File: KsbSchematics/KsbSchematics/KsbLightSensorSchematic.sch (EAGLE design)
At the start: 30 parts, among them IC1 7805L, IC2 LM311N, U1 ATTINY84

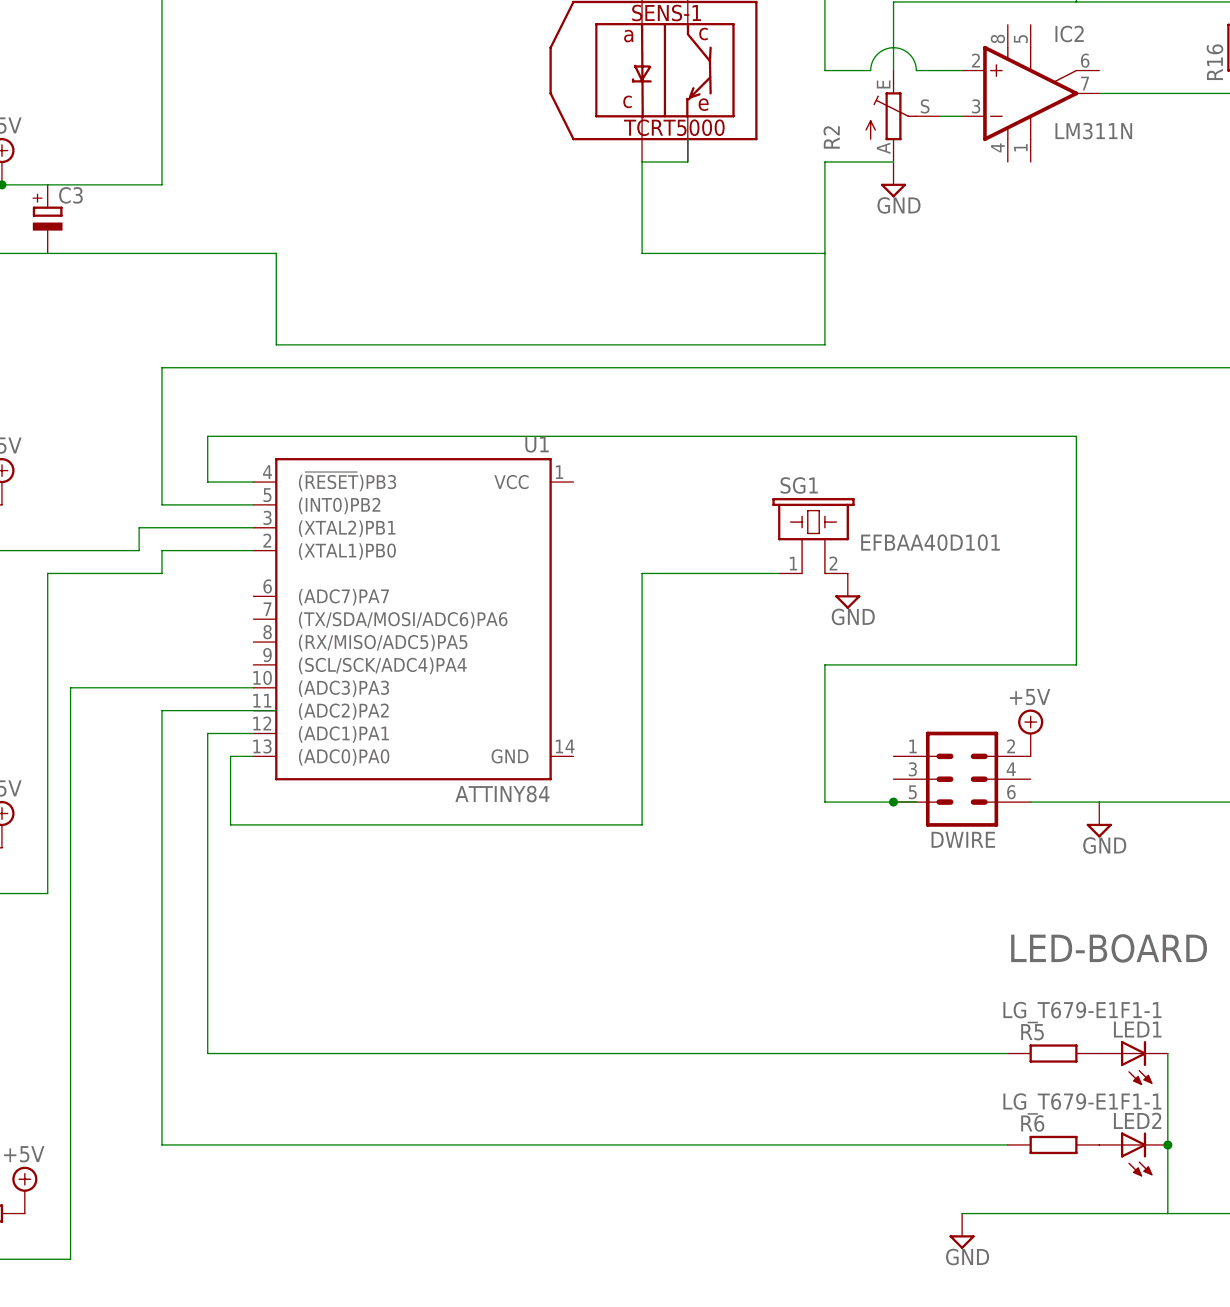
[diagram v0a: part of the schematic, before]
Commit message: schematic changes
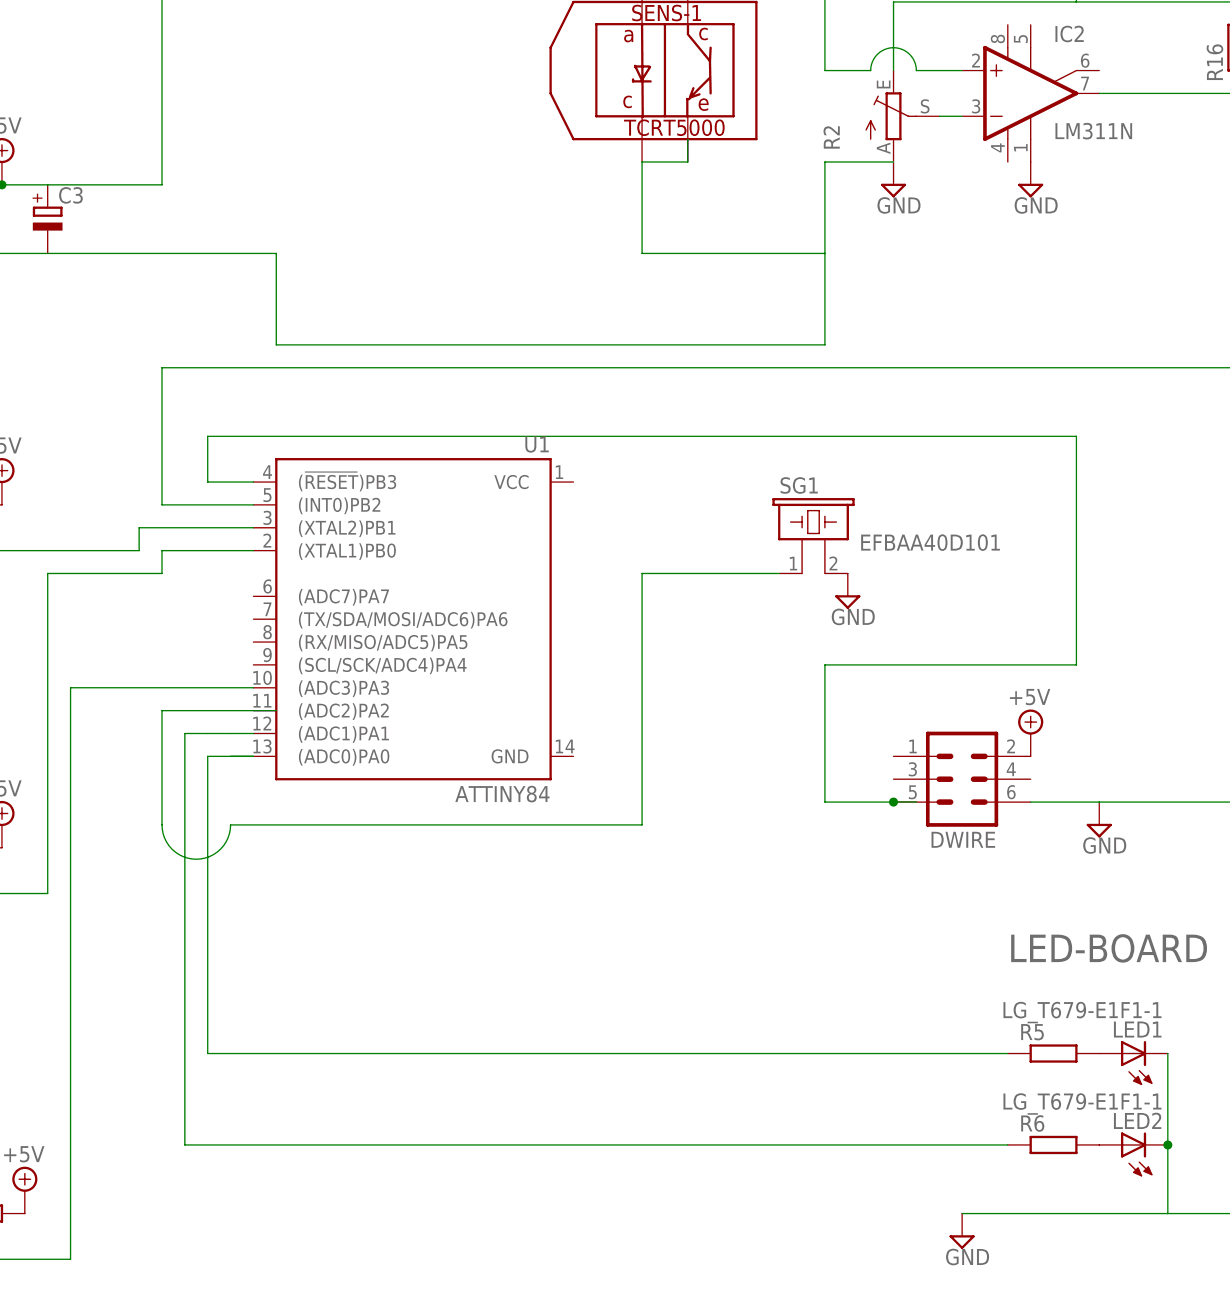
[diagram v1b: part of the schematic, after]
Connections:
- removed net N$10: R6.1
- removed net N$19: SG1.1, U1.(ADC0)PA0
- new net N$12: R6.1, U1.(ADC1)PA1
- new net N$14: SG1.1
- net GND: now also IC2.GND
- net LED-BOARD: now also U1.(ADC0)PA0; no longer U1.(ADC1)PA1
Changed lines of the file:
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@@
 <part name="R7" library="resistor" deviceset="R-EU_" device="0613/5V" value="2k"/>
 <part name="R8" library="resistor" deviceset="R-EU_" device="0613/5V" value="2k"/>
+<part name="SUPPLY26" library="supply2" deviceset="GND" device=""/>
 </parts>
 <sheets>
@@
 <instance part="R7" gate="G$1" x="132.08" y="157.48"/>
 <instance part="R8" gate="G$1" x="132.08" y="149.86"/>
+<instance part="SUPPLY26" gate="GND" x="132.08" y="124.46"/>
 </instances>
 <busses>
@@
 <pinref part="SUPPLY17" gate="GND" pin="GND"/>
 </segment>
+<segment>
+<pinref part="IC2" gate="A" pin="GND"/>
+<pinref part="SUPPLY26" gate="GND" pin="GND"/>
+</segment>
 </net>
 <net name="N$6" class="0">
@@
 </segment>
 </net>
-<net name="N$10" class="0">
-<segment>
-<wire x1="35.56" y1="17.78" x2="129.54" y2="17.78" width="0.1524" layer="91"/>
-<pinref part="R6" gate="G$1" pin="1"/>
-<wire x1="35.56" y1="17.78" x2="35.56" y2="66.04" width="0.1524" layer="91"/>
-<wire x1="35.56" y1="66.04" x2="48.26" y2="66.04" width="0.1524" layer="91"/>
-</segment>
-</net>
 <net name="LED-BOARD" class="0">
 <segment>
@@
 <pinref part="R5" gate="G$1" pin="1"/>
 <label x="129.54" y="38.1" size="3.048" layer="95"/>
-<wire x1="40.64" y1="27.94" x2="40.64" y2="63.5" width="0.1524" layer="91"/>
-<pinref part="U1" gate="U1" pin="(ADC1)PA1"/>
-<wire x1="40.64" y1="63.5" x2="45.72" y2="63.5" width="0.1524" layer="91"/>
+<wire x1="40.64" y1="27.94" x2="40.64" y2="60.96" width="0.1524" layer="91"/>
+<pinref part="U1" gate="U1" pin="(ADC0)PA0"/>
+<wire x1="43.18" y1="60.96" x2="45.72" y2="60.96" width="0.1524" layer="91"/>
+<wire x1="40.64" y1="60.96" x2="45.72" y2="60.96" width="0.1524" layer="91"/>
 </segment>
 </net>
@@
 <pinref part="S2" gate="1" pin="O"/>
 <label x="-76.2" y="50.8" size="2.54" layer="95" rot="R180"/>
-</segment>
-</net>
-<net name="N$19" class="0">
-<segment>
-<pinref part="SG1" gate="G$1" pin="1"/>
-<wire x1="104.14" y1="81.28" x2="88.9" y2="81.28" width="0.1524" layer="91"/>
-<wire x1="88.9" y1="81.28" x2="88.9" y2="53.34" width="0.1524" layer="91"/>
-<wire x1="88.9" y1="53.34" x2="43.18" y2="53.34" width="0.1524" layer="91"/>
-<wire x1="43.18" y1="53.34" x2="43.18" y2="60.96" width="0.1524" layer="91"/>
-<pinref part="U1" gate="U1" pin="(ADC0)PA0"/>
-<wire x1="43.18" y1="60.96" x2="45.72" y2="60.96" width="0.1524" layer="91"/>
 </segment>
 </net>
@@
 </segment>
 </net>
+<net name="N$12" class="0">
+<segment>
+<pinref part="U1" gate="U1" pin="(ADC1)PA1"/>
+<wire x1="38.1" y1="63.5" x2="40.64" y2="63.5" width="0.1524" layer="91"/>
+<pinref part="R6" gate="G$1" pin="1"/>
+<wire x1="43.18" y1="63.5" x2="45.72" y2="63.5" width="0.1524" layer="91"/>
+<wire x1="129.54" y1="17.78" x2="38.1" y2="17.78" width="0.1524" layer="91"/>
+<wire x1="38.1" y1="17.78" x2="38.1" y2="63.5" width="0.1524" layer="91"/>
+<wire x1="40.64" y1="63.5" x2="43.18" y2="63.5" width="0.1524" layer="91"/>
+</segment>
+</net>
+<net name="N$14" class="0">
+<segment>
+<wire x1="35.56" y1="66.04" x2="48.26" y2="66.04" width="0.1524" layer="91"/>
+<pinref part="SG1" gate="G$1" pin="1"/>
+<wire x1="104.14" y1="81.28" x2="88.9" y2="81.28" width="0.1524" layer="91"/>
+<wire x1="88.9" y1="81.28" x2="88.9" y2="53.34" width="0.1524" layer="91"/>
+<wire x1="88.9" y1="53.34" x2="43.18" y2="53.34" width="0.1524" layer="91"/>
+<wire x1="43.18" y1="53.34" x2="35.56" y2="53.34" width="0.1524" layer="91" curve="-180"/>
+<wire x1="35.56" y1="66.04" x2="35.56" y2="53.34" width="0.1524" layer="91"/>
+</segment>
+</net>
